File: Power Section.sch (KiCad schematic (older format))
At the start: 21 parts, among them J1 BATT, J17 CK-JS102011SAQN, Q1 IRLML9301TRPBF, Q7 IRLML9301TRPBF, U1 LM1117LDX, U2 LM1117LDX

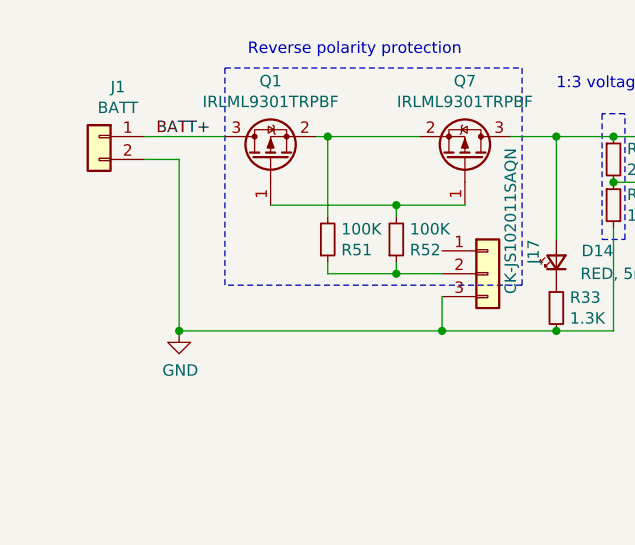
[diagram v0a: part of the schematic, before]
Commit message: Holy $hi3t
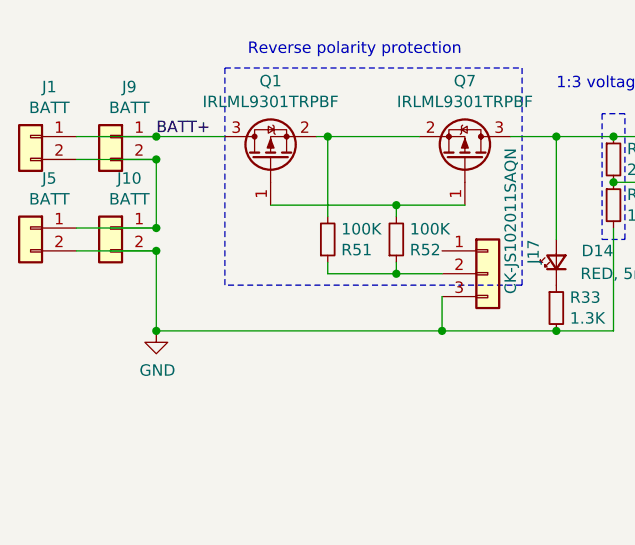
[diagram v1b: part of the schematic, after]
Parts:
- added J10, J5, J9: BATT, Connector_PinHeader_2.54mm:PinHeader_1x02_P2.54mm_Vertical, symbol Connector_Generic:Conn_01x02
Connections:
- net BATT+: now also J9.1 (Pin_1)
- net GND: now also J10.2 (Pin_2), J5.2 (Pin_2); no longer J1.2 (Pin_2)
- new net: J1.2 (Pin_2), J10.1 (Pin_1), J5.1 (Pin_1), J9.2 (Pin_2)
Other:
- moved on the sheet: J1
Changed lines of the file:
@@
 L Connector_Generic:Conn_01x02 J1
 U 1 1 5E80D37A
-P 1550 2700
-F 0 "J1" H 1468 2917 50  0000 C CNN
-F 1 "BATT" H 1468 2826 50  0000 C CNN
-F 2 "Connector_PinHeader_2.54mm:PinHeader_1x02_P2.54mm_Vertical" H 1550 2700 50  0001 C CNN
-F 3 "~" H 1550 2700 50  0001 C CNN
-	1    1550 2700
+P 1250 2700
+F 0 "J1" H 1168 2917 50  0000 C CNN
+F 1 "BATT" H 1168 2826 50  0000 C CNN
+F 2 "Connector_PinHeader_2.54mm:PinHeader_1x02_P2.54mm_Vertical" H 1250 2700 50  0001 C CNN
+F 3 "~" H 1250 2700 50  0001 C CNN
+	1    1250 2700
 	-1   0    0    -1
 $EndComp
-Wire Wire Line
-	1750 2800 1900 2800
 Wire Wire Line
 	3800 2900 4200 2900
@@
 L power:GND #PWR0195
 U 1 1 5E892532
-P 1900 3550
-F 0 "#PWR0195" H 1900 3300 50  0001 C CNN
-F 1 "GND" H 1905 3377 50  0000 C CNN
-F 2 "" H 1900 3550 50  0001 C CNN
-F 3 "" H 1900 3550 50  0001 C CNN
-	1    1900 3550
+P 1800 3550
+F 0 "#PWR0195" H 1800 3300 50  0001 C CNN
+F 1 "GND" H 1805 3377 50  0000 C CNN
+F 2 "" H 1800 3550 50  0001 C CNN
+F 3 "" H 1800 3550 50  0001 C CNN
+	1    1800 3550
 	1    0    0    -1
 $EndComp
@@
 	1    0    0    1
 $EndComp
-Wire Wire Line
-	2100 2700 1750 2700
 $Comp
 L Device:R_Small R51
@@
 $EndComp
 Wire Wire Line
-	1900 2800 1900 3550
-Wire Wire Line
 	3800 3100 3800 3550
-Connection ~ 1900 3550
+Connection ~ 1800 3550
 Wire Wire Line
 	3050 3400 3050 3550
 Wire Wire Line
 	3050 3550 3550 3550
-Wire Wire Line
-	1900 3550 3050 3550
-Connection ~ 3050 3550
 Wire Wire Line
 	3350 2700 3550 2700
@@
 Text Notes 3550 2500 0    50   ~ 0
 1:3 voltage divider
+$Comp
+L Connector_Generic:Conn_01x02 J5
+U 1 1 5F9516BF
+P 1250 3100
+F 0 "J5" H 1168 3317 50  0000 C CNN
+F 1 "BATT" H 1168 3226 50  0000 C CNN
+F 2 "Connector_PinHeader_2.54mm:PinHeader_1x02_P2.54mm_Vertical" H 1250 3100 50  0001 C CNN
+F 3 "~" H 1250 3100 50  0001 C CNN
+	1    1250 3100
+	-1   0    0    -1
+$EndComp
+$Comp
+L Connector_Generic:Conn_01x02 J9
+U 1 1 5F956258
+P 1600 2700
+F 0 "J9" H 1518 2917 50  0000 C CNN
+F 1 "BATT" H 1518 2826 50  0000 C CNN
+F 2 "Connector_PinHeader_2.54mm:PinHeader_1x02_P2.54mm_Vertical" H 1600 2700 50  0001 C CNN
+F 3 "~" H 1600 2700 50  0001 C CNN
+	1    1600 2700
+	-1   0    0    -1
+$EndComp
+$Comp
+L Connector_Generic:Conn_01x02 J10
+U 1 1 5F95794D
+P 1600 3100
+F 0 "J10" H 1518 3317 50  0000 C CNN
+F 1 "BATT" H 1518 3226 50  0000 C CNN
+F 2 "Connector_PinHeader_2.54mm:PinHeader_1x02_P2.54mm_Vertical" H 1600 3100 50  0001 C CNN
+F 3 "~" H 1600 3100 50  0001 C CNN
+	1    1600 3100
+	-1   0    0    -1
+$EndComp
+Wire Wire Line
+	1450 2700 1800 2700
+Connection ~ 1800 2700
+Wire Wire Line
+	1450 2800 1800 2800
+Wire Wire Line
+	1800 2800 1800 3100
+Connection ~ 1800 2800
+Wire Wire Line
+	1450 3100 1800 3100
+Connection ~ 1800 3100
+Wire Wire Line
+	1450 3200 1800 3200
+Connection ~ 1800 3200
+Wire Wire Line
+	1800 3200 1800 3550
+Wire Wire Line
+	1800 2700 2100 2700
+Wire Wire Line
+	1800 3550 3050 3550
+Connection ~ 3050 3550
 $EndSCHEMATC
